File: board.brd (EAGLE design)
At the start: 49.2 x 21.6 mm, 4 parts

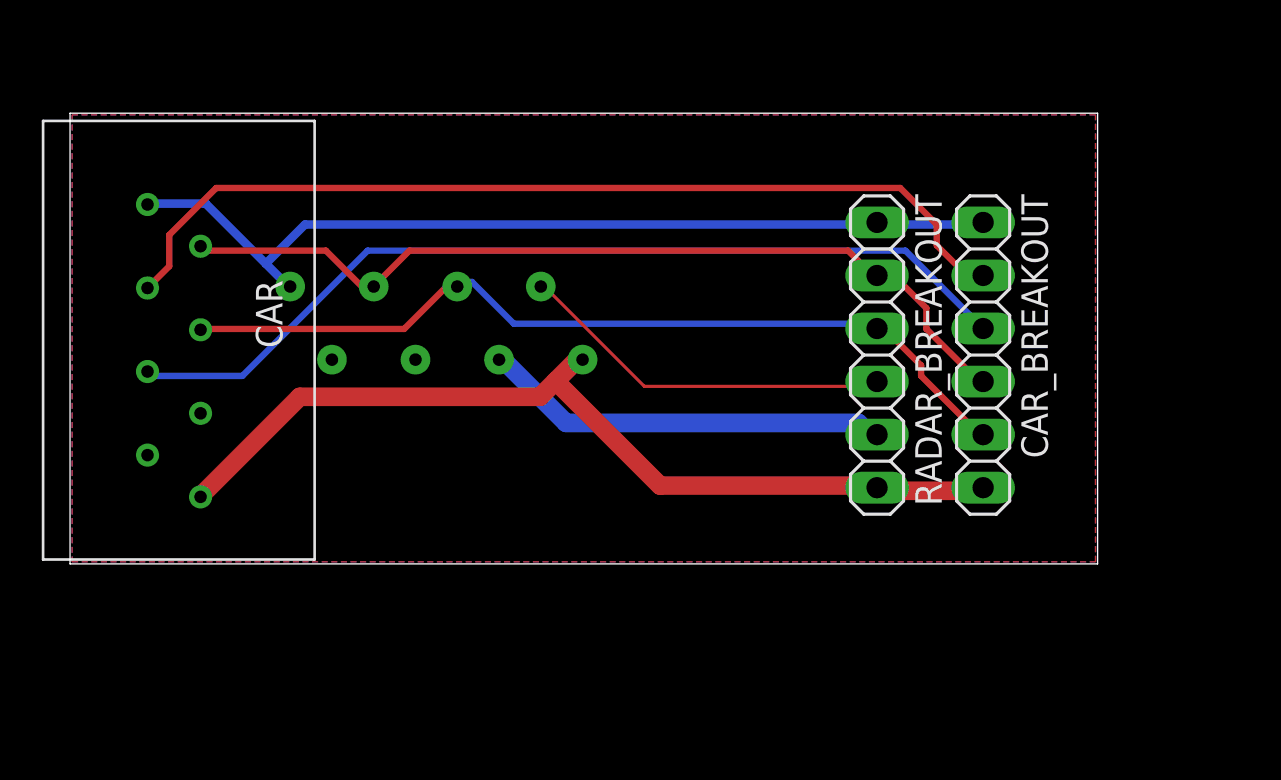
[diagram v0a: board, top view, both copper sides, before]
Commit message: v1
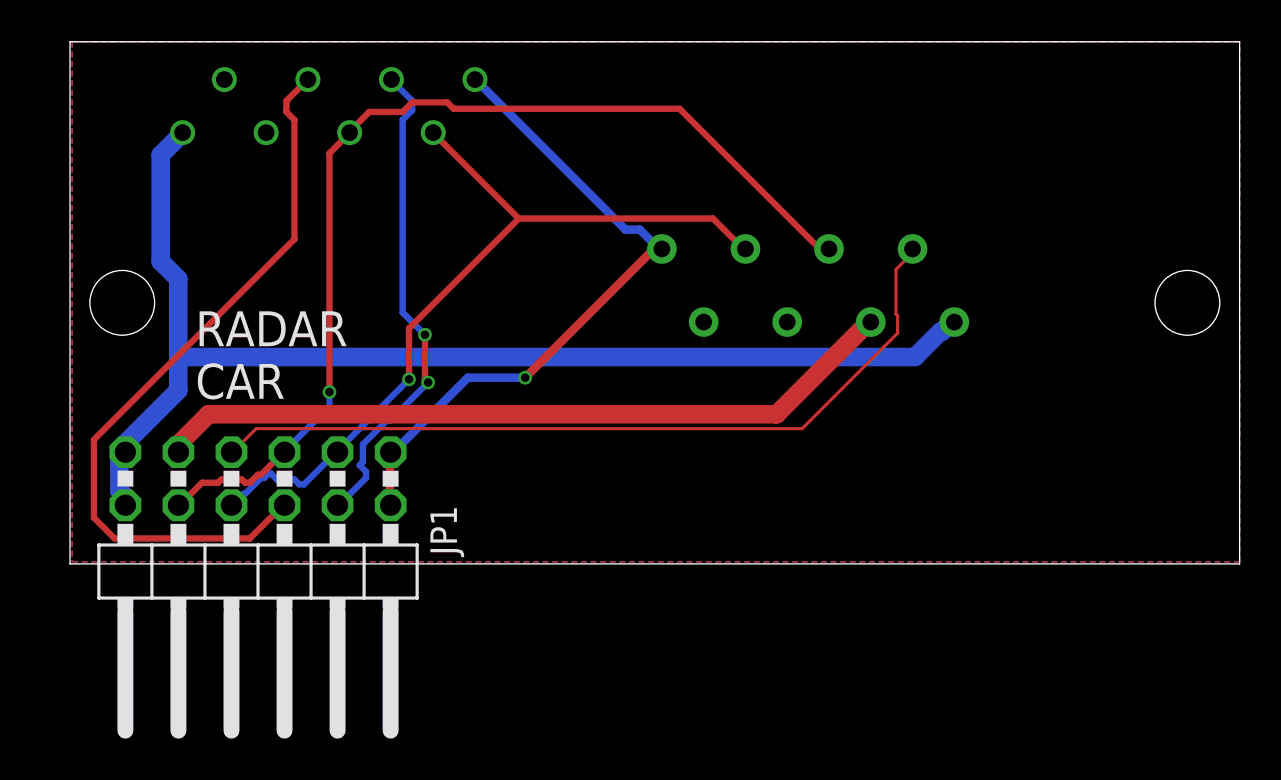
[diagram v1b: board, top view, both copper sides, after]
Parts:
- removed CAR_BREAKOUT, RADAR_BREAKOUT: (no value), pinhead:1X06
- added JP1: (no value), pinhead:2X06/90
- moved RADAR 17.9 mm to (36.3, 15.1)
- moved CAR 7.02 mm to (7.39, 23.2), flipped to the bottom, turned to 180 degrees
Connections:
- net FCAN_H_P: now also JP1.4; no longer CAR_BREAKOUT.2
- net FCAN_L_N: now also JP1.6; no longer CAR_BREAKOUT.3
- net GND: now also JP1.1, JP1.2; no longer CAR_BREAKOUT.1, RADAR_BREAKOUT.1
- net HTR: now also JP1.9; no longer RADAR_BREAKOUT.5
- net IGN: now also JP1.11, JP1.12; no longer CAR_BREAKOUT.6, RADAR_BREAKOUT.6
- net TESLACAN_H_P: now also JP1.3, JP1.8; no longer CAR_BREAKOUT.4, RADAR_BREAKOUT.2
- net TESLACAN_L_N: now also JP1.10, JP1.5; no longer CAR_BREAKOUT.5, RADAR_BREAKOUT.3
- net WAU: now also JP1.7; no longer RADAR_BREAKOUT.4
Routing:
- net FCAN_H_P: track 45.2 -> 23.7 mm, vias 0 -> 2
- net WAU: track 18.2 -> 38.6 mm
- net HTR: track 19.8 -> 36.0 mm
- net IGN: track 44.0 -> 57.8 mm
- net GND: track 43.7 -> 32.0 mm, vias 0 -> 1
- net FCAN_L_N: track 44.2 -> 35.7 mm
- net TESLACAN_L_N: track 42.0 -> 49.3 mm, vias 0 -> 1
- net TESLACAN_H_P: track 42.3 -> 38.8 mm, vias 0 -> 1
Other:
- board size 49.2 x 21.6 mm -> 56 x 25 mm
- board text added: "RADAR CAR"
- board text added: "Tesla Radar > Honda Bosch csouers 2019 github.com/csouers/tesladapter"
